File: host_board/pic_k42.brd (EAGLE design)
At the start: 55.6 x 67.3 mm, 39 parts, among them IC1 PIC18F57K42-E_PT, IC2 REF3440IDBVR, IC3 MAX232, K1 G6K-2P, Q1 ASF1, X1 332-02, X2 332-02, X3 332-02, X4 22-23-2101, X5 22-23-2101, X6 22-23-2101, X7 22-23-2101

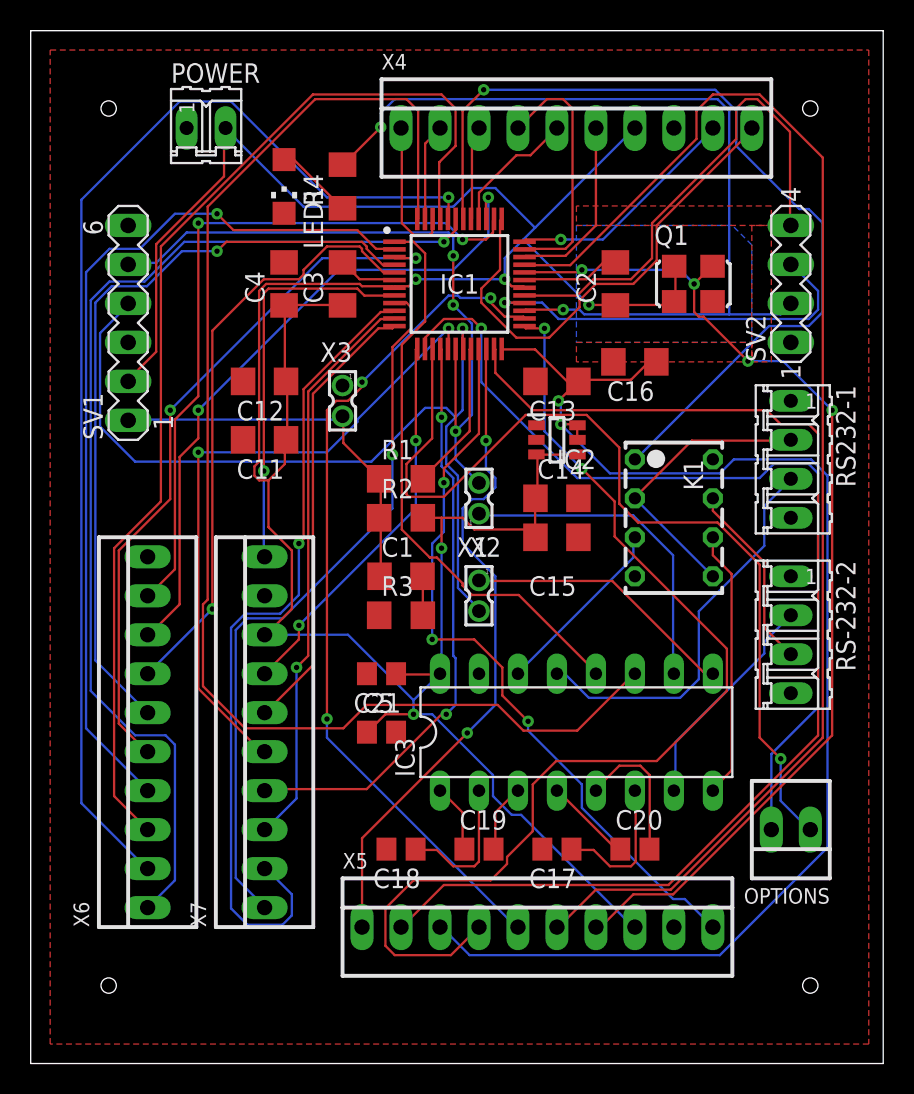
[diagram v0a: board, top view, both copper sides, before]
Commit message: update
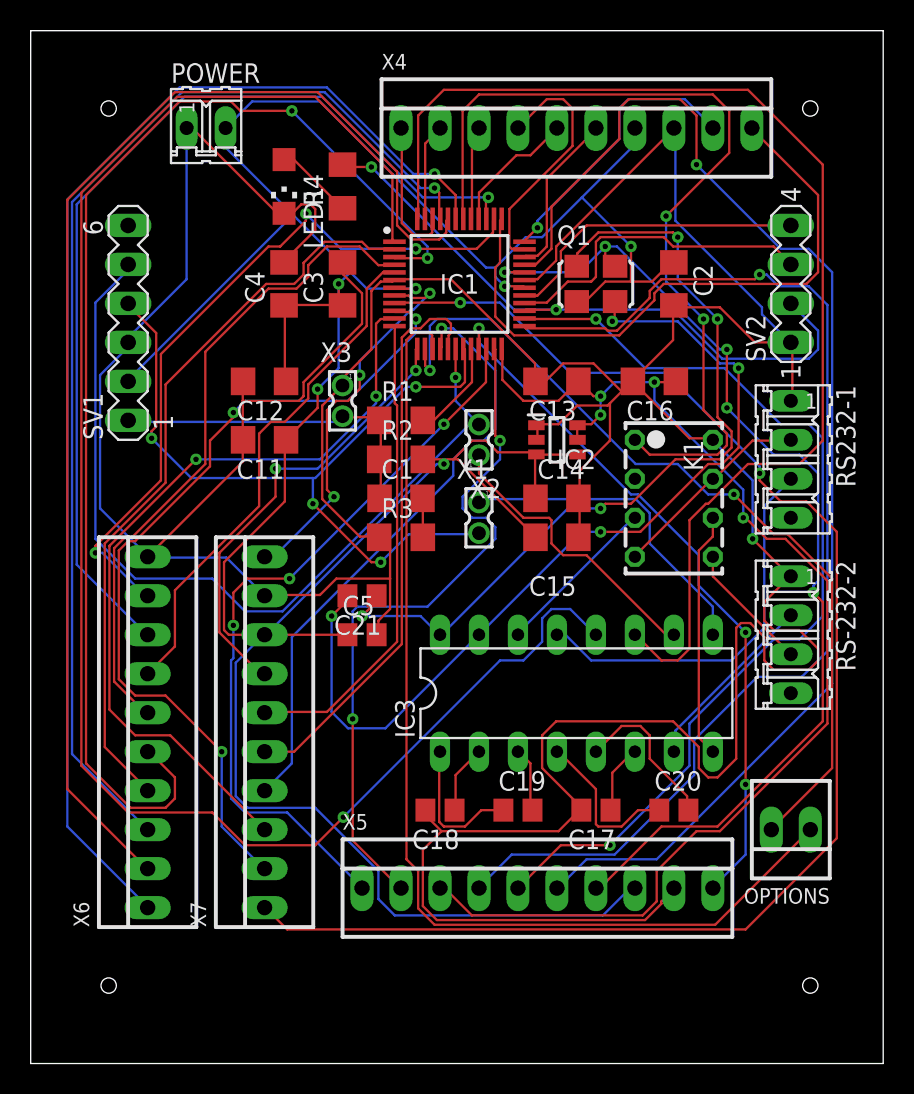
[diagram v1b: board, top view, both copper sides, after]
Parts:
- moved C5 6.48 mm to (45.7, 19.1)
- moved Q1 6.35 mm to (61.0, 41.9)
- moved C21 5.24 mm to (45.7, 21.6)
- moved C1 5.08 mm to (48.3, 27.9)
- moved X1 5.08 mm to (53.3, 26.7)
- moved R3 5.08 mm to (48.3, 25.4)
- moved C2 3.81 mm to (66.0, 41.9), turned to 270 degrees
- moved R1 3.81 mm to (48.3, 33.0)
- moved R2 3.81 mm to (48.3, 30.5)
- moved X2 3.81 mm to (53.3, 31.8)
- moved C20 3.59 mm to (66.0, 7.62)
- moved C17 3.59 mm to (61.0, 7.62)
- moved C18 3.59 mm to (50.8, 7.62)
- moved C19 3.59 mm to (55.9, 7.62)
- moved IC3 2.54 mm to (59.7, 15.2)
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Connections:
- removed net N$17: K1.7, RS-232-2.3
- new net GND: C21.2, IC3.15, Q1.2
- new net N$62: K1.5, RS-232-2.3
- new net VCC: C21.1, IC3.16, Q1.4
- net N$14: now also K1.4, K1.7; no longer K1.2, K1.5
- net VDD: no longer C21.1, IC3.16, Q1.4
- net VSS: no longer C21.2, IC3.15, Q1.2
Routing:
- net VSS: track 10.2 -> 309.8 mm, vias 0 -> 1
- net N$18: track 37.6 -> 110.4 mm, vias 0 -> 1
- net GND: track 0.00 -> 58.6 mm, vias 0 -> 4
- net VCC: track 0.00 -> 54.6 mm, vias 0 -> 4
- net N$53: track 47.2 -> 95.9 mm, vias 1 -> 2
- net N$47: track 46.0 -> 79.8 mm
- net N$37: track 76.3 -> 45.6 mm, vias 0 -> 2
- net N$51: track 43.6 -> 63.9 mm, vias 2 -> 1
- net N$23: track 58.9 -> 42.3 mm
- net VDD: track 197.7 -> 213.3 mm, vias 5 -> 6
- net N$55: track 37.3 -> 51.8 mm, vias 1 -> 2
- net N$17: track 12.3 -> 0.00 mm
- net N$25: track 32.1 -> 20.1 mm
- net N$7: track 45.2 -> 56.6 mm, vias 3 -> 1
- net N$43: track 70.1 -> 81.1 mm
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- removed copper zone on layer 1, net VSS
- removed copper zone on layer 16, net VSS
